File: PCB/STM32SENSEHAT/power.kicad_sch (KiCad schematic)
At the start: 26 parts, among them Q1 FS8205A, U1 MCP1700x-330xxTT, U11 AO3401A_C306862, U2 DW01A, U7 TP4056

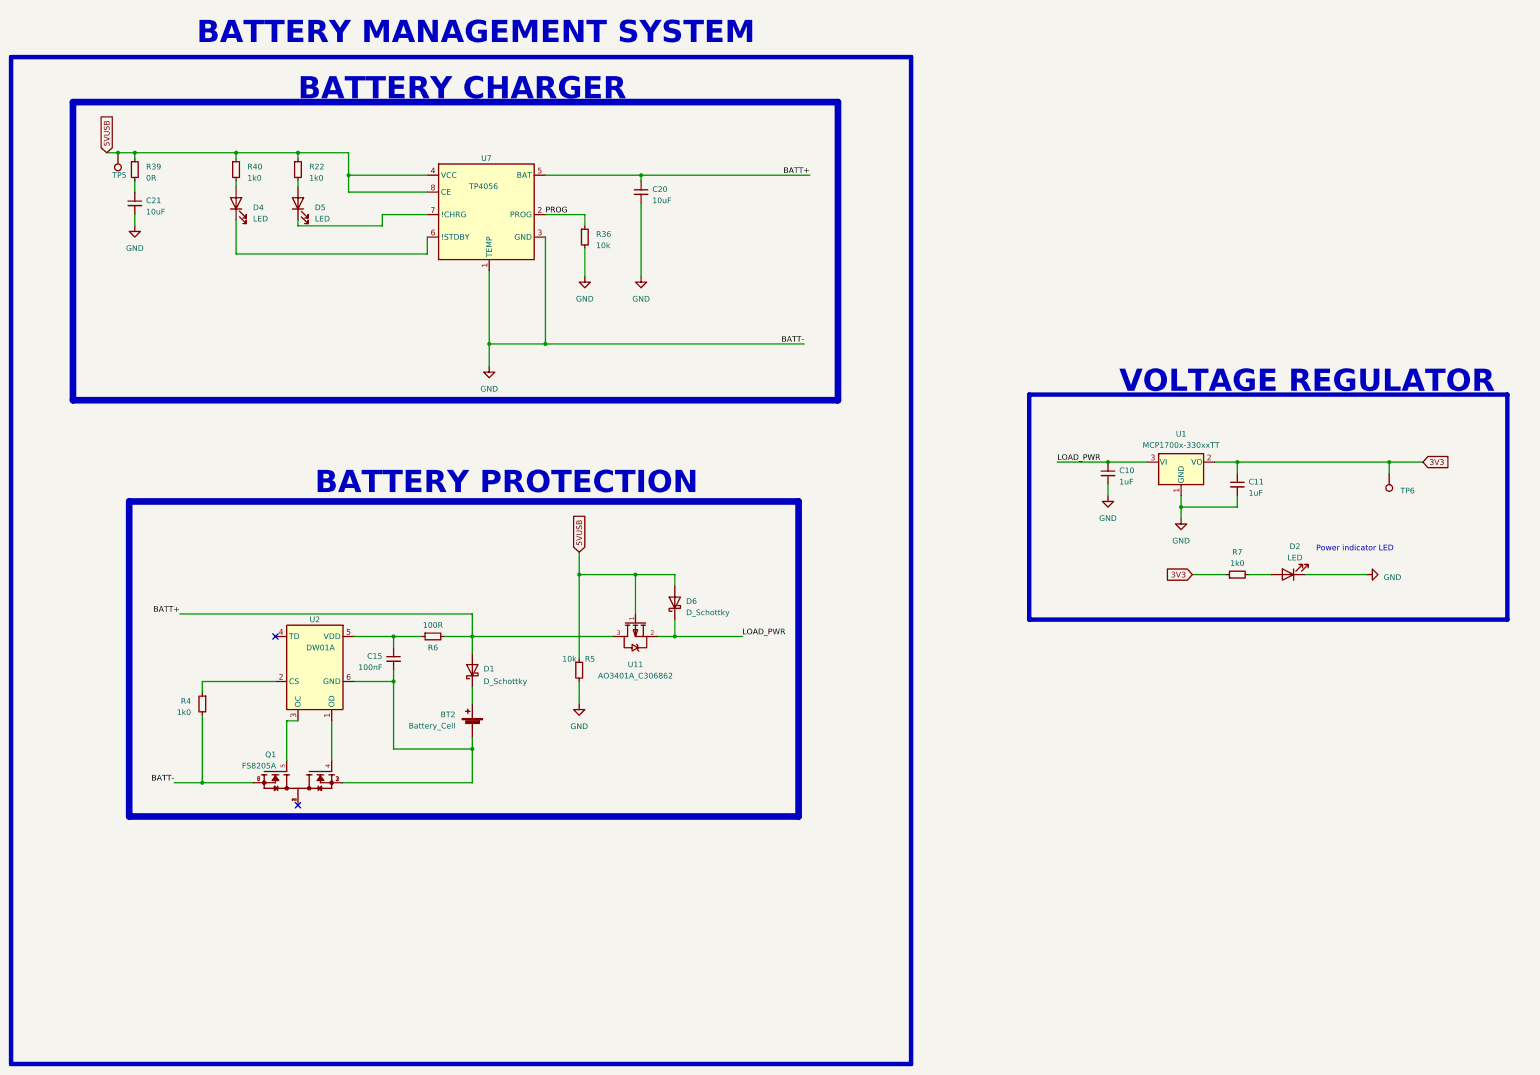
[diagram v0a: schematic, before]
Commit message: Last change
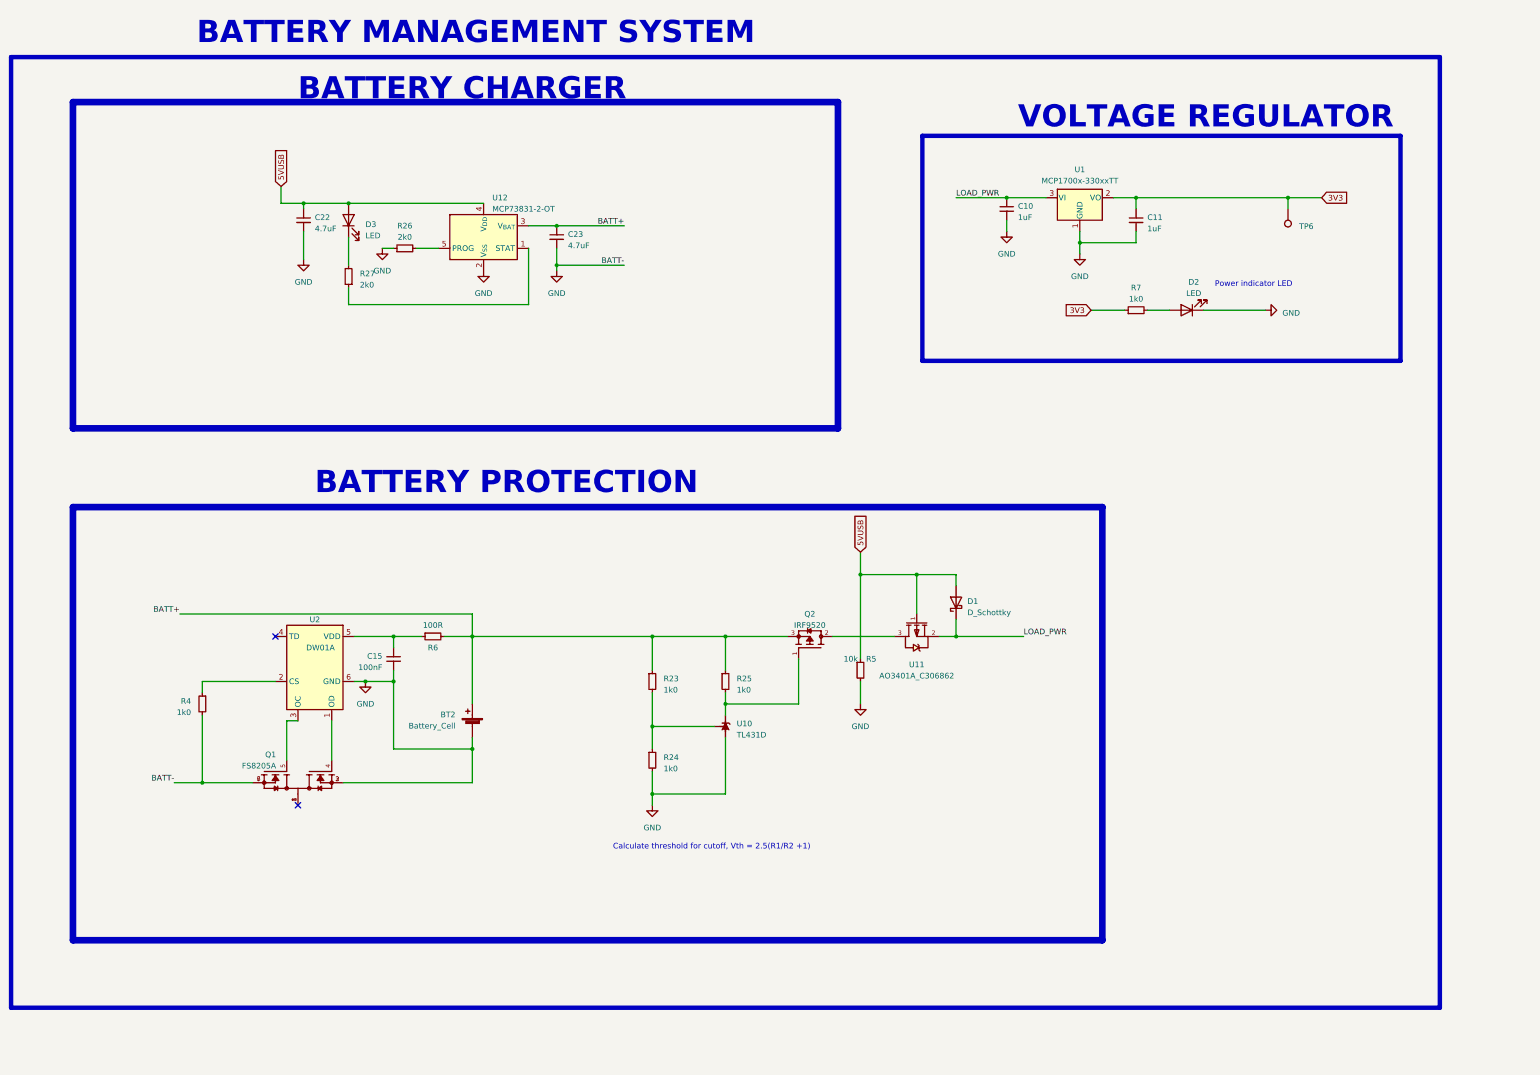
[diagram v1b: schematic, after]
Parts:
- removed C20, C21: 10uF, Capacitor_SMD:C_0805_2012Metric, symbol Device:C_Small
- removed D4, D5: LED, LED_THT:LED_D5.0mm, symbol Device:LED
- removed D6: D_Schottky, JLCfootprint:SOT-23-3_L3.0-W1.7-P0.95-LS2.9-BR, symbol Device:D_Schottky
- removed R22, R40: 1k0, Resistor_SMD:R_0805_2012Metric, symbol Device:R_Small
- removed R36: 10k, Resistor_SMD:R_0805_2012Metric, symbol Device:R_Small
- removed R39: 0R, Resistor_SMD:R_0805_2012Metric, symbol Device:R_Small
- removed TP5: TestPoint, TestPoint:TestPoint_Pad_D3.0mm, symbol Connector:TestPoint
- removed U7: TP4056, JLCfootprint:ESOP-8_L4.9-W3.9-P1.27-LS6.0-BL-EP, symbol UCT:TP4056
- added C22, C23: 4.7uF, Capacitor_SMD:C_0805_2012Metric, symbol Device:C_Small
- added D3: LED, LED_THT:LED_D5.0mm, symbol Device:LED
- added Q2: IRF9520, TO254P1052X465X1989-3, symbol IRF9520:IRF9520
- added R23, R24, R25: 1k0, Resistor_SMD:R_0805_2012Metric, symbol Device:R_Small
- added R26, R27: 2k0, Resistor_SMD:R_0805_2012Metric, symbol Device:R_Small
- added U10: TL431D, Package_SO:SOIC-8_3.9x4.9mm_P1.27mm, symbol Reference_Voltage:TL431D
- added U12: MCP73831-2-OT, Package_TO_SOT_SMD:SOT-23-5, symbol Battery_Management:MCP73831-2-OT
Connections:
- net 5VUSB: now also D1.2 (A), C22.1, D3.2 (A), U12.4 (V_{DD})
- net BATT+: now also BT2.1 (+), C23.1, Q2.3, R23.1, R25.1, U12.3 (V_{BAT}); no longer D1.2 (A), U11.3 (D)
- net GND: now also BT2.2 (-), C15.2, Q1.2, Q1.3, U2.6 (GND), C22.2, C23.2, R24.2, R26.1, U10.2 (A), U10.3 (A), U10.6 (A), U10.7 (A), U12.2 (V_{SS})
- net LOAD_PWR: now also D1.1 (K)
- new net: R27.1, U12.1 (STAT)
- new net: D3.1 (K), R27.2
- new net: Q2.1, R25.2, U10.1 (K)
- new net: Q2.2, U11.3 (D)
- new net: R23.2, R24.1, U10.8 (REF)
- new net: R26.2, U12.5 (PROG)
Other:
- note added: "Calculate threshold for cutoff, Vth = 2.5(R1/R2 +1)"
- moved on the sheet: C10, C11, D2, R7, TP6, U1
